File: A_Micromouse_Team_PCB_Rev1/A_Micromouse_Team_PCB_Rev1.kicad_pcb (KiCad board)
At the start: 2 copper layers, 13 parts, among them J1 Conn_01x07_Pin, J10 Conn_01x06, J2 Conn_01x07_Pin, J3 Conn_01x07_Pin, J4 Conn_01x07_Pin, J5 Conn_01x06_Pin, J6 Conn_01x06_Pin, J7 Conn_01x04_Socket, J8 Conn_01x07_Pin, J9 Conn_01x02_Socket, U1 Teensy4.0, U2 BNO055, U3 TB6612FNG

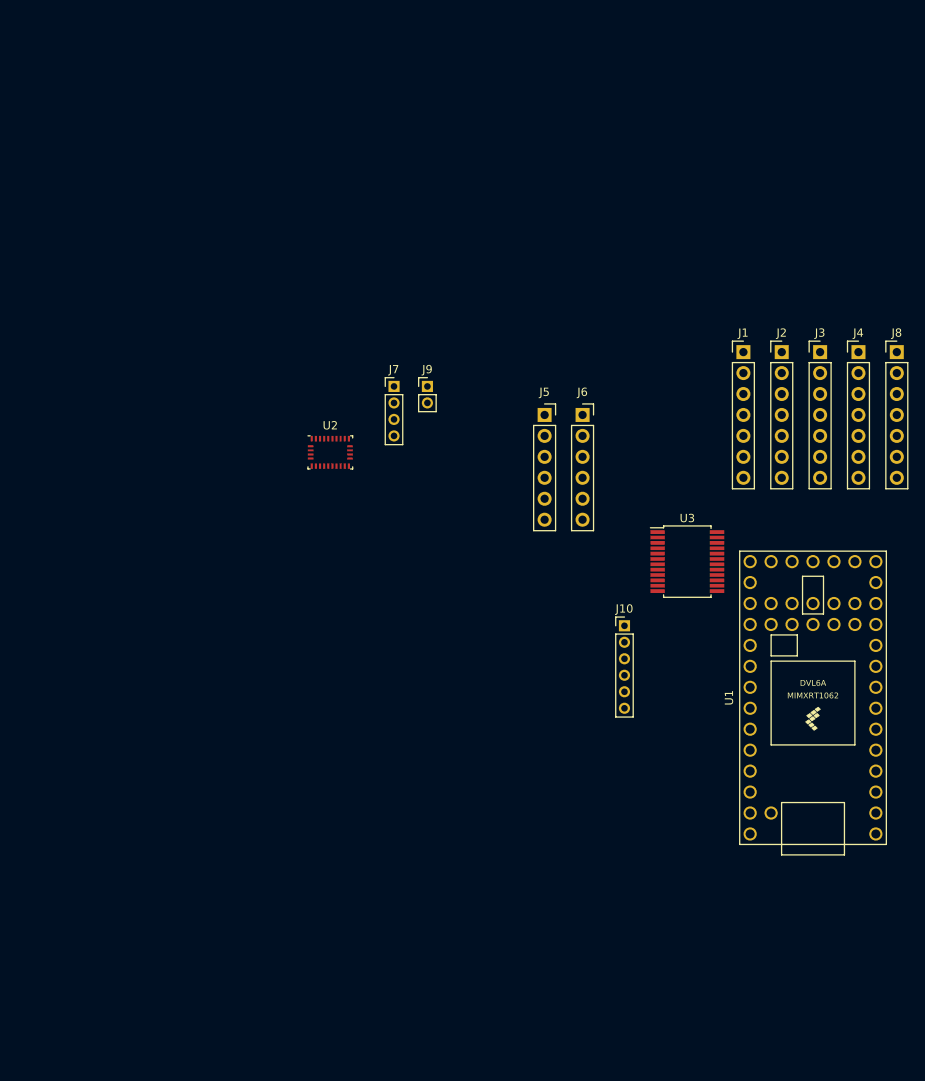
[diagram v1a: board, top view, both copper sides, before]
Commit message: checked all footprints and created a max footprint
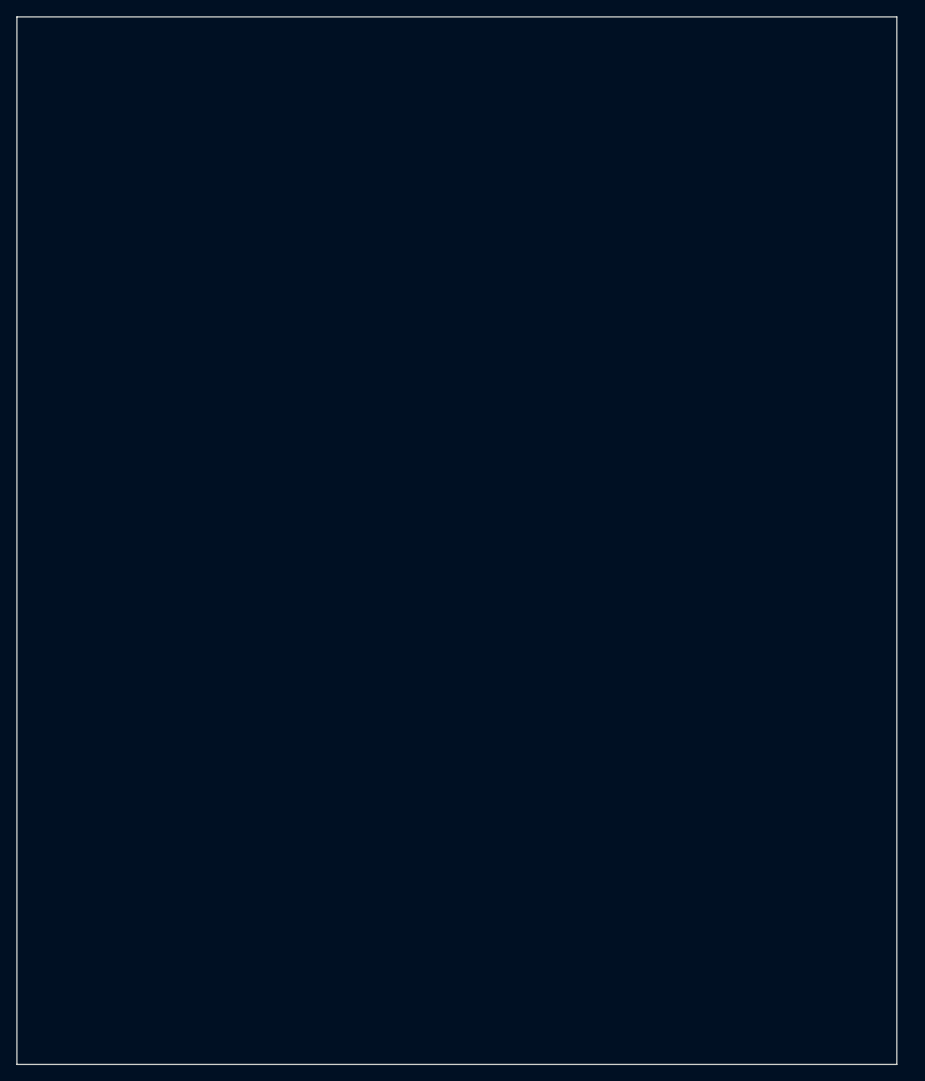
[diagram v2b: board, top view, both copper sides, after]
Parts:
- removed J1, J2, J3, J4, J8: Conn_01x07_Pin, Connector_PinHeader_2.54mm:PinHeader_1x07_P2.54mm_Vertical
- removed J10: Conn_01x06, Connector_PinHeader_2.00mm:PinHeader_1x06_P2.00mm_Vertical
- removed J5, J6: Conn_01x06_Pin, Connector_PinSocket_2.54mm:PinSocket_1x06_P2.54mm_Vertical
- removed J7: Conn_01x04_Socket, Connector_PinHeader_2.00mm:PinHeader_1x04_P2.00mm_Vertical
- removed J9: Conn_01x02_Socket, Connector_PinHeader_2.00mm:PinHeader_1x02_P2.00mm_Vertical
- removed U1: Teensy4.0, Teensy4.0:Teensy40
- removed U2: BNO055, Package_LGA:LGA-28_5.2x3.8mm_P0.5mm
- removed U3: TB6612FNG, Package_SO:SSOP-24_5.3x8.2mm_P0.65mm
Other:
- board outline added: 106.7 x 127 mm
